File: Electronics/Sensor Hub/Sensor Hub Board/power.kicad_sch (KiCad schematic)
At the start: 26 parts, among them IC201 TPS563202DRLR, IC202 TPS563202DRLR, J203 Pluggable_Terminal_01x02, Q201 DMP3028LFDE

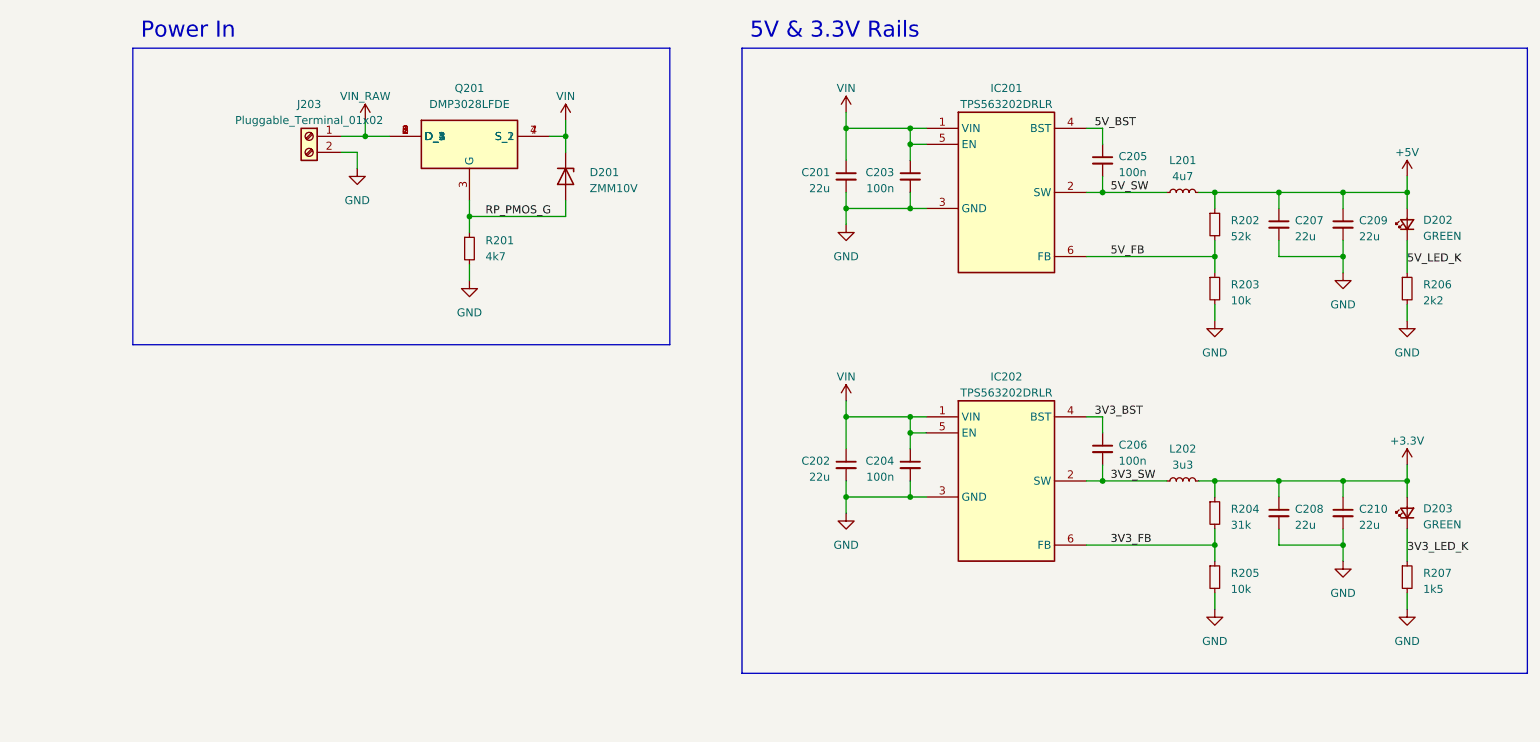
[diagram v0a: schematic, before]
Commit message: All boards done
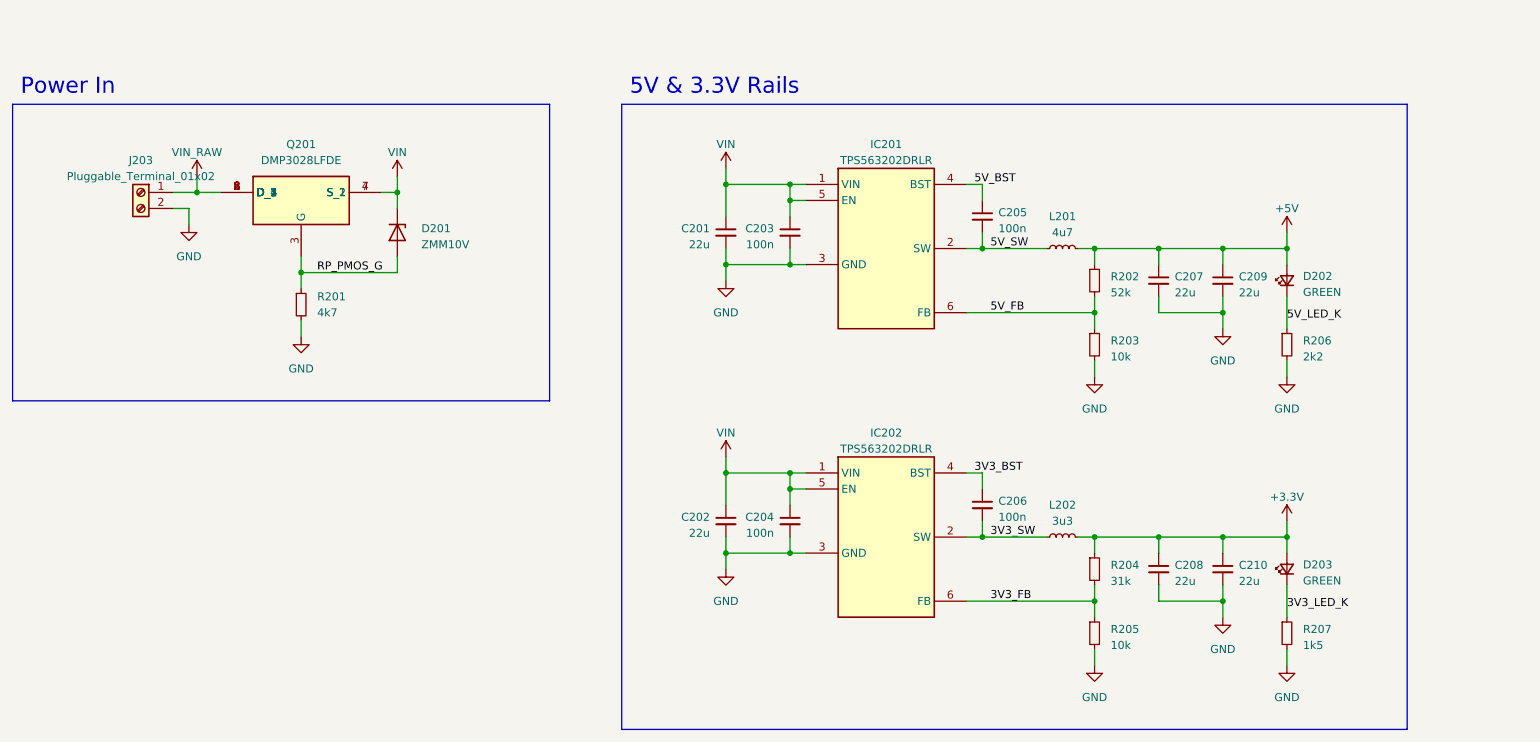
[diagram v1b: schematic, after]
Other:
- moved on the sheet: C201, C202, C203, C204, C205, C206, C207, C208, C209, C210, D201, D202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
